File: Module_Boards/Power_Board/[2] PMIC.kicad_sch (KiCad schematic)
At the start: 24 parts, among them U2 MAX77654MENV+T

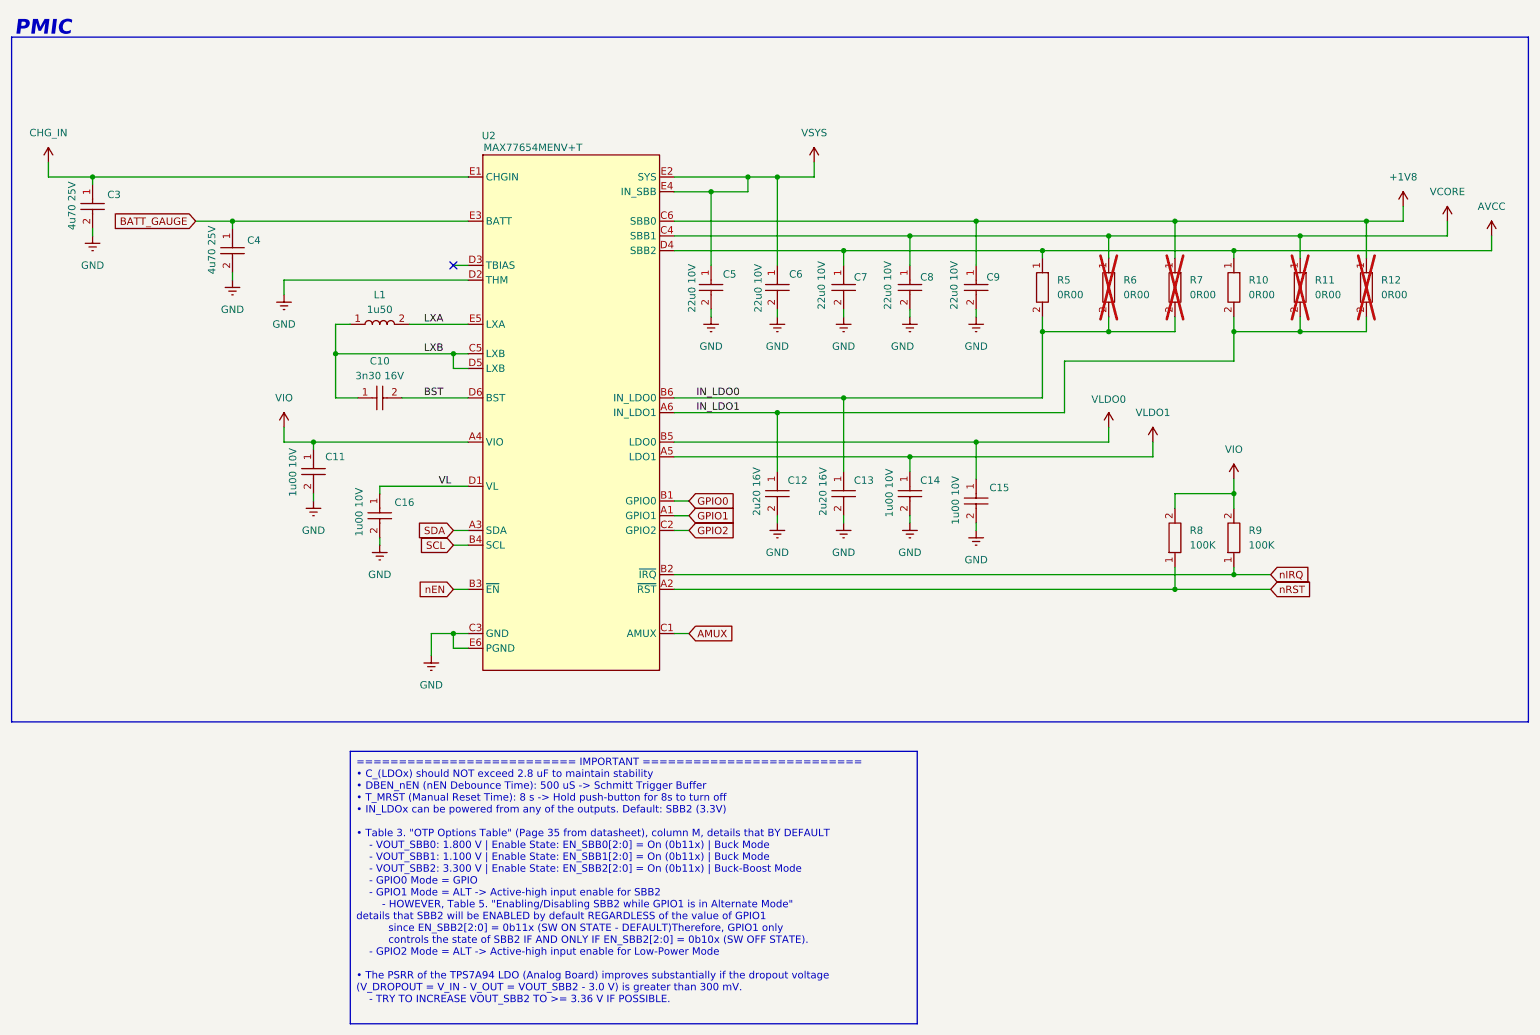
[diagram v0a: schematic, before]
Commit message: Push with updated readme
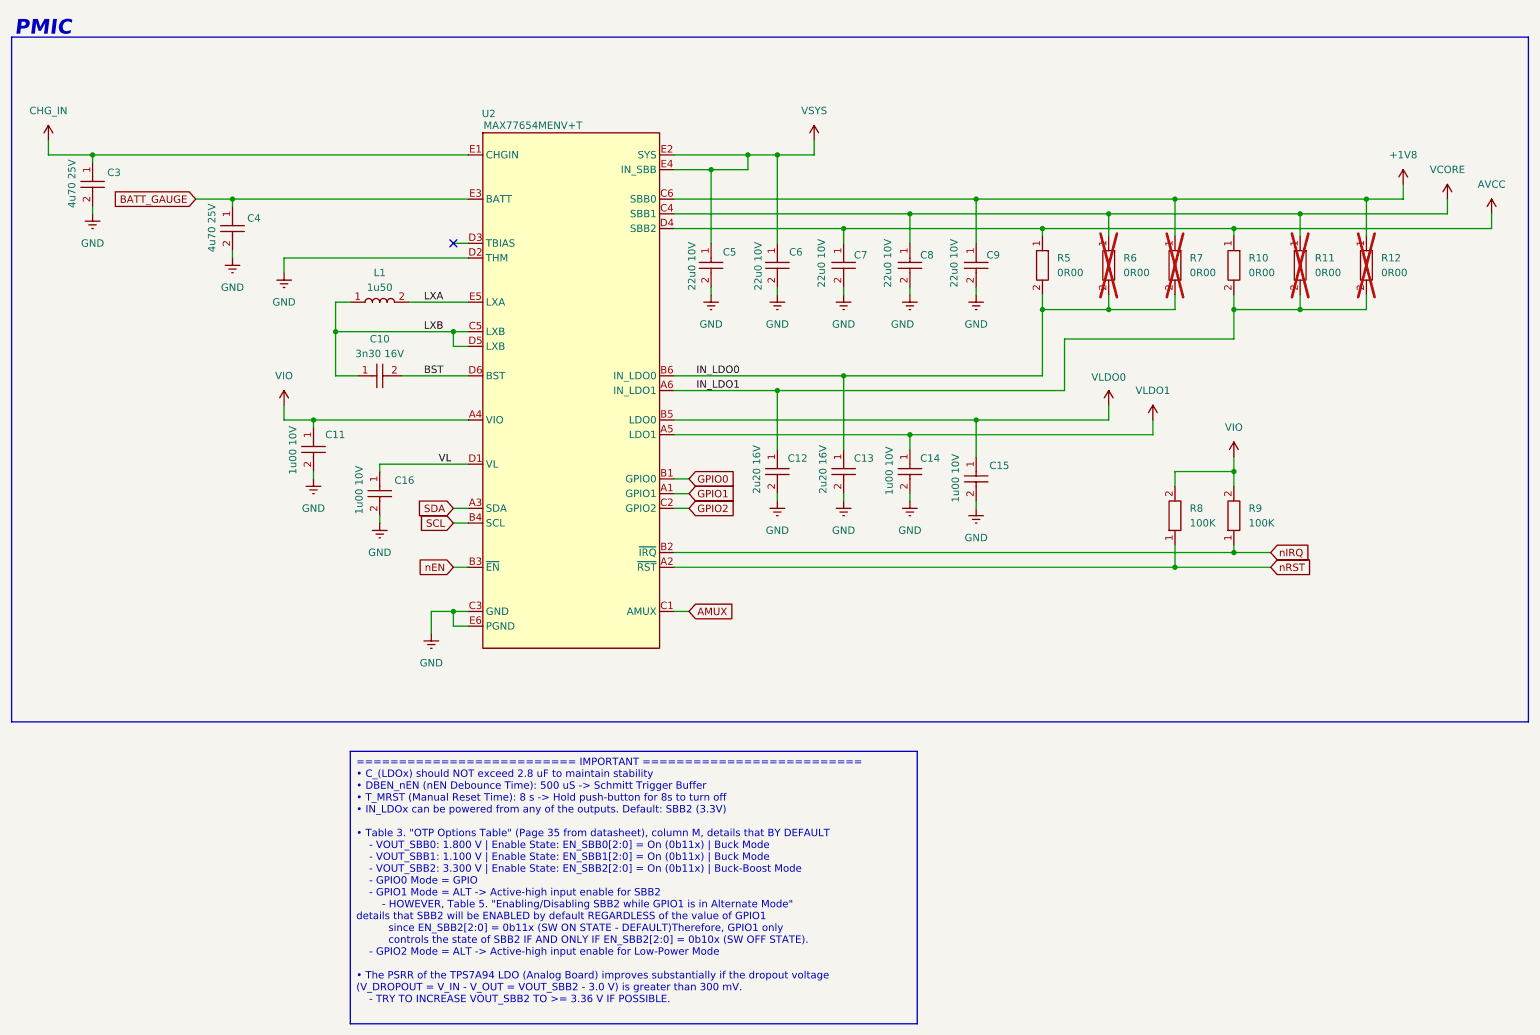
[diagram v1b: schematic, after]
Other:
- moved on the sheet: C10, C11, C12, C13, C14, C15, C16, C3, C4, C5, C6, C7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
